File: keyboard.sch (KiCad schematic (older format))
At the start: 23 parts, among them IC1 ATMEGA32U4, P1 CONN_3X2, P2 DIL24, X1 ASX3F

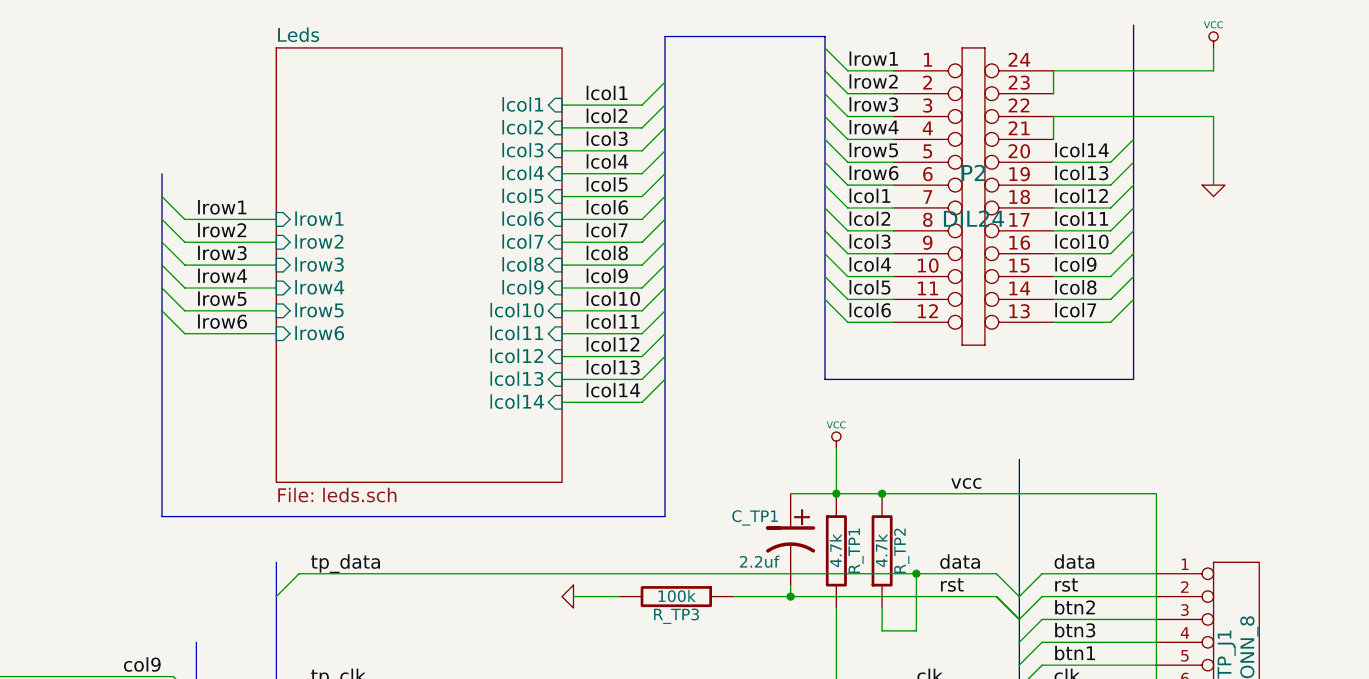
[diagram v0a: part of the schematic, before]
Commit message: 一些改动
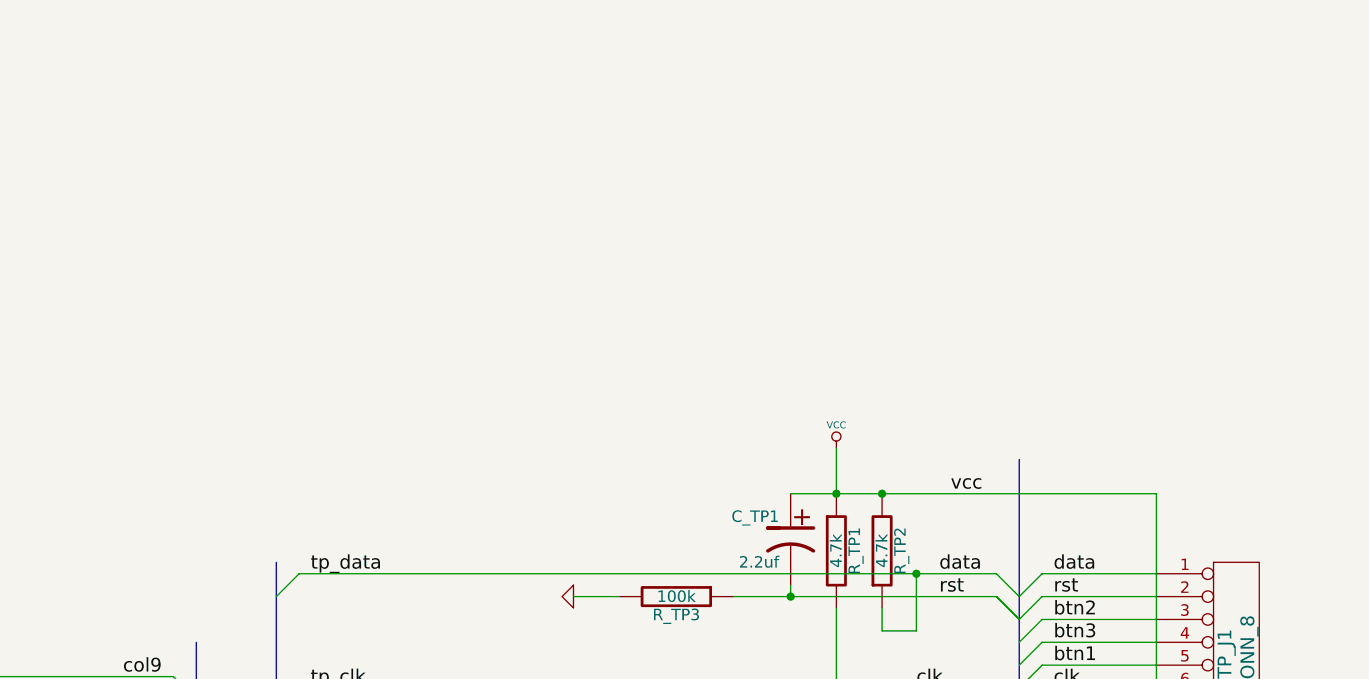
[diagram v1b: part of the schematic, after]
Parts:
- removed P2: DIL24, connectors:ffc-0.5mm-24p, symbol DIL24
